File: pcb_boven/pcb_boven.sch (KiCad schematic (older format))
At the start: 30 parts, among them U1 miniIMU-9_v6, U2 openMV_M7_R2

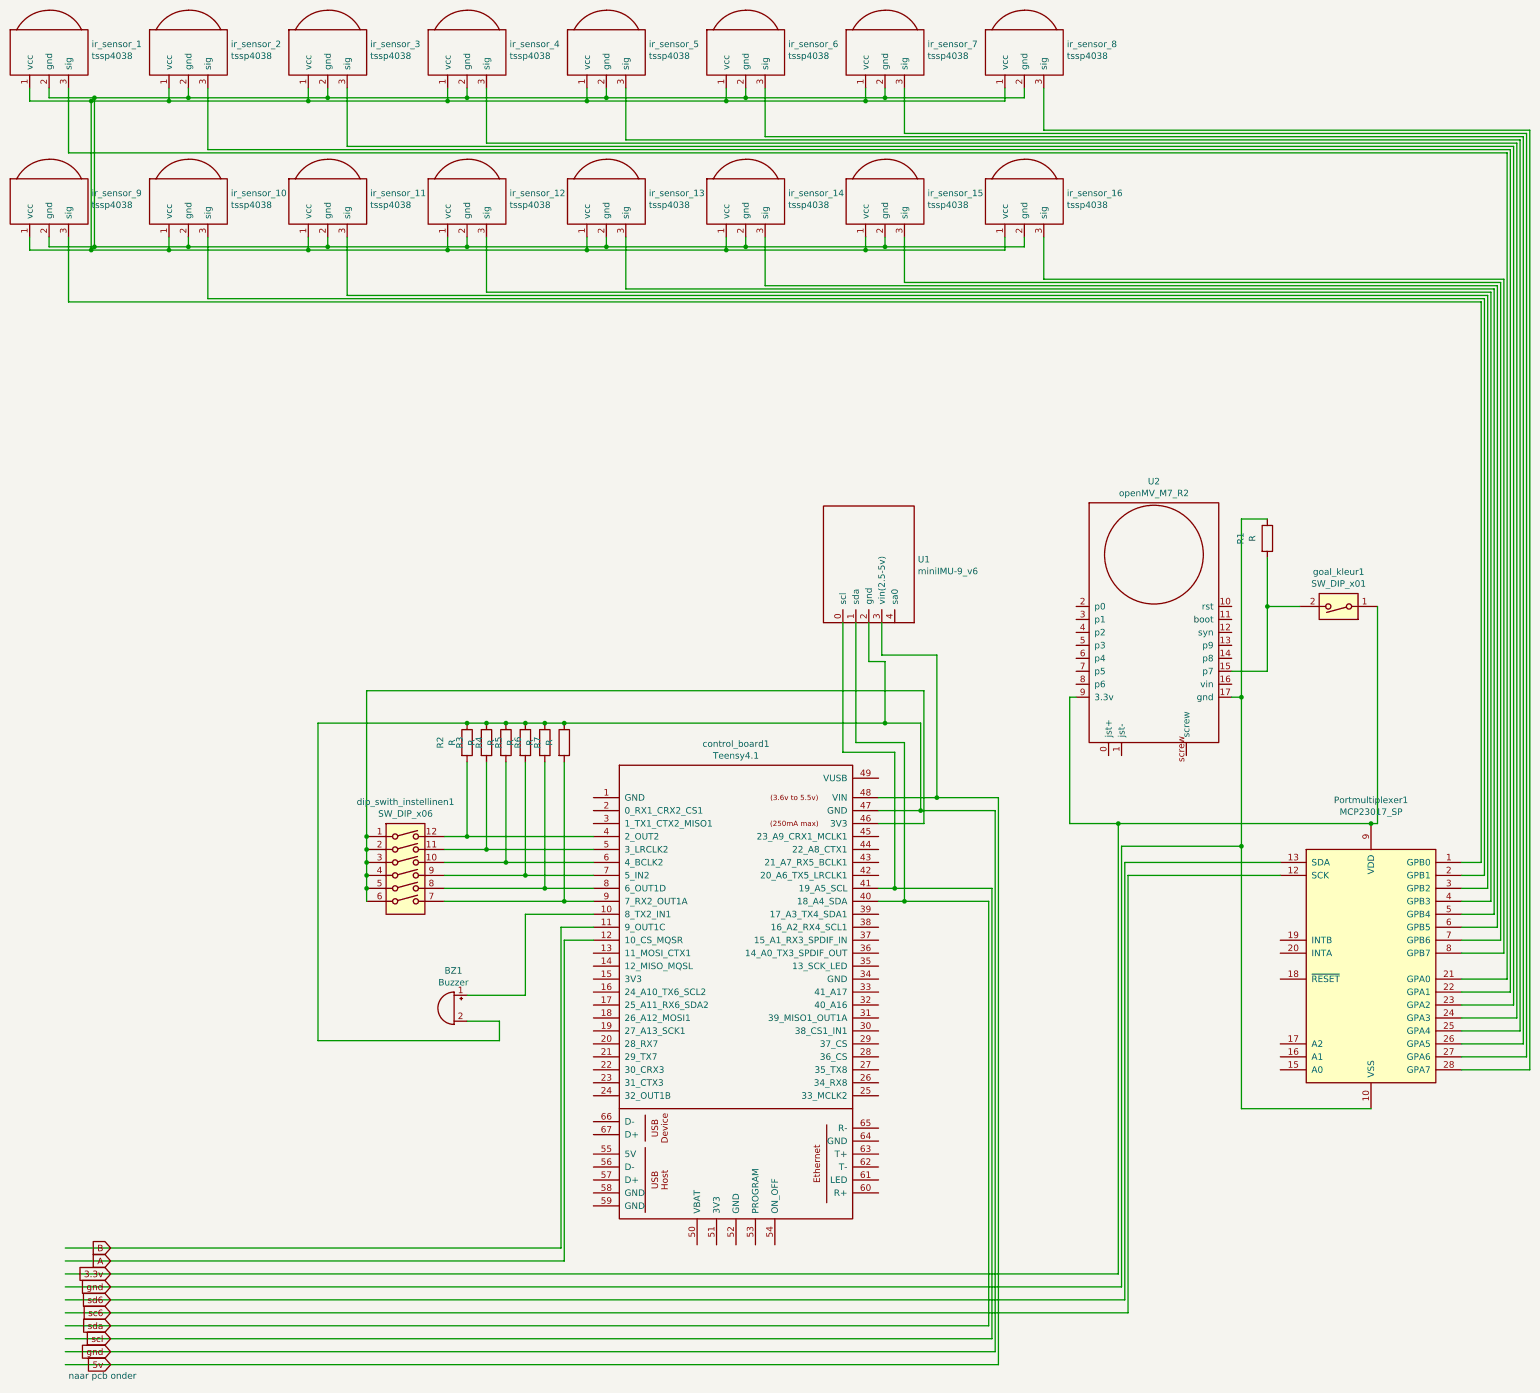
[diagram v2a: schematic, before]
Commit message: pcb onder gemaakt
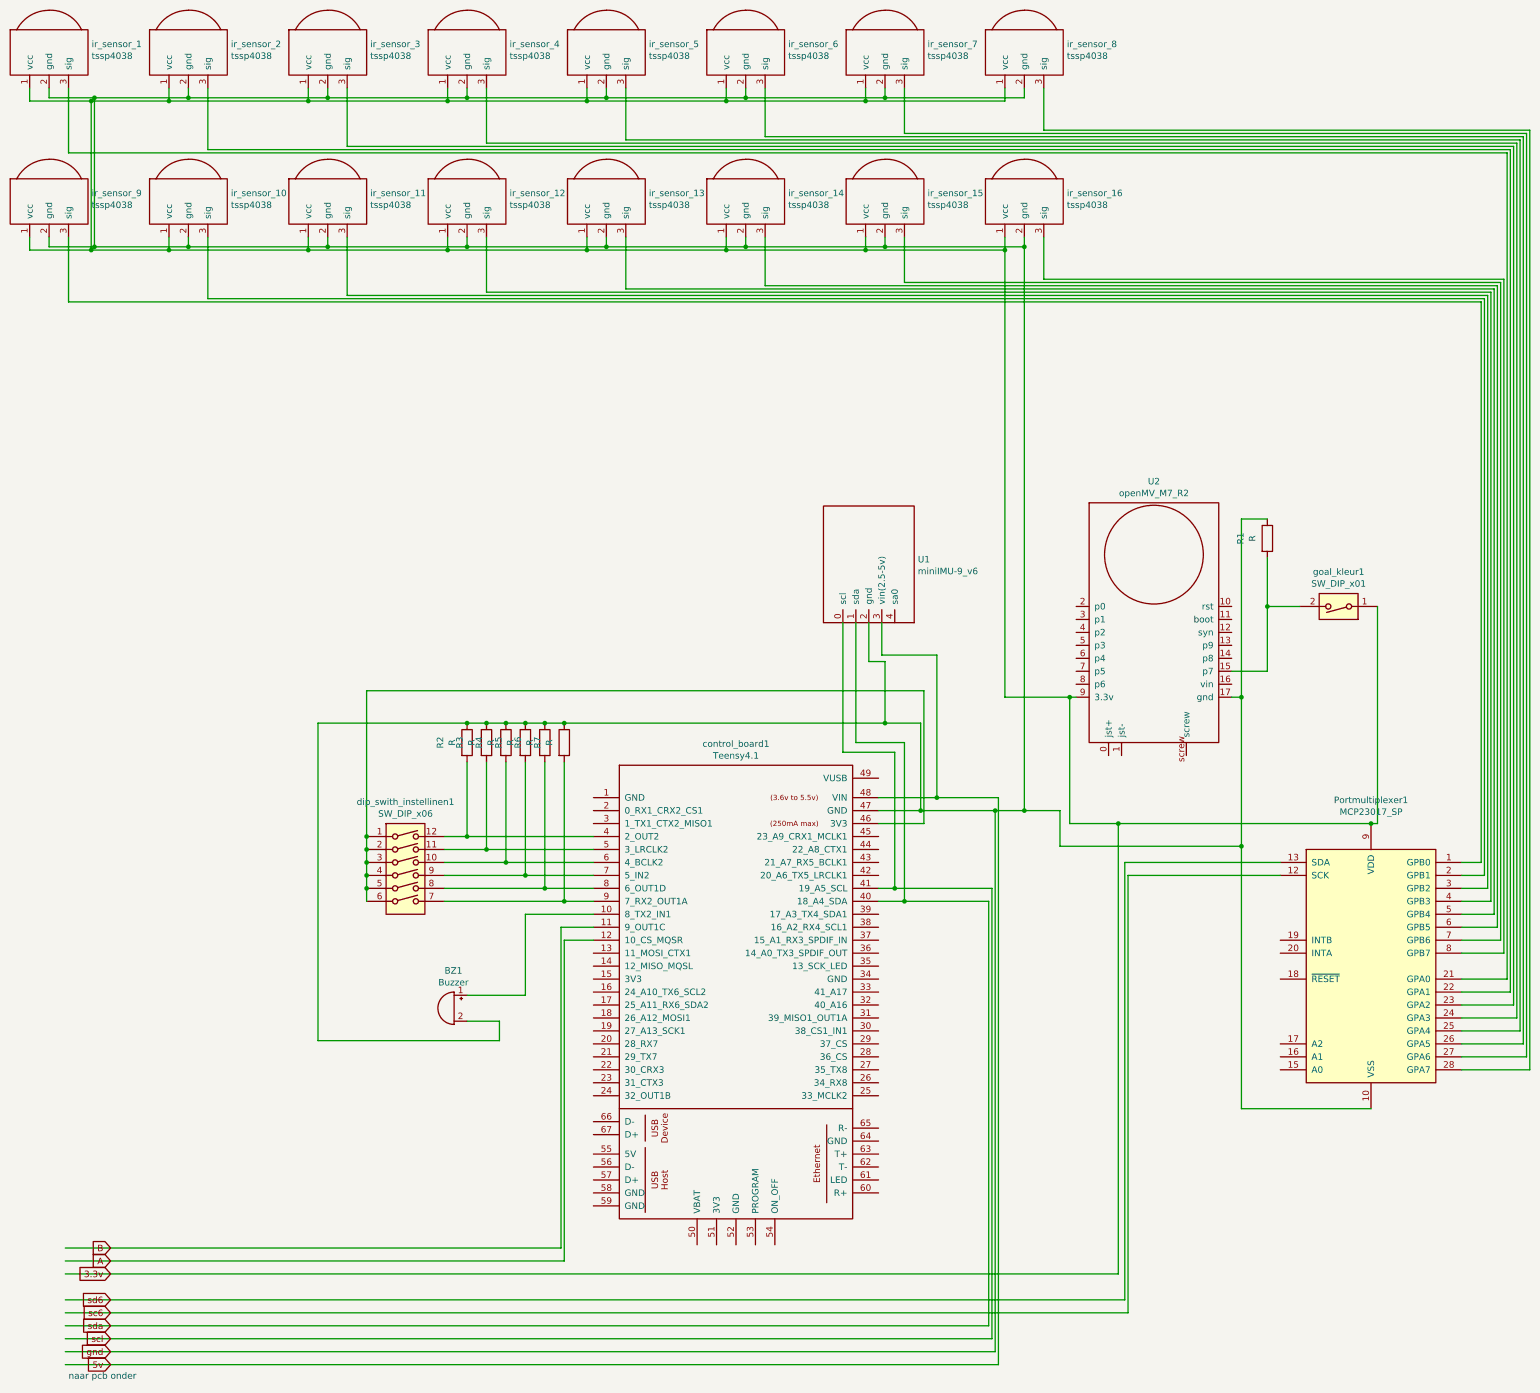
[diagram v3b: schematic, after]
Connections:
- wire segments 234 -> 238
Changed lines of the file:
@@
 	10025 5825 10025 6975
-Wire Wire Line
-	10025 6975 9100 6975
-Wire Wire Line
-	9100 6975 9100 10375
-Wire Wire Line
-	9100 10375 950  10375
 Wire Wire Line
 	9075 10275 9075 6800
@@
 Text GLabel 1300 10275 0    50   Input ~ 0
 3.3v
-Text GLabel 1300 10375 0    50   Input ~ 0
-gnd
 Wire Wire Line
 	11025 6800 9075 6800
@@
 Wire Wire Line
 	4775 10075 950  10075
+Wire Wire Line
+	8125 6700 8350 6700
+Wire Wire Line
+	8625 6700 8625 6975
+Wire Wire Line
+	8625 6975 10025 6975
+Connection ~ 8125 6700
+Wire Wire Line
+	8350 2350 8350 6700
+Connection ~ 8350 2350
+Connection ~ 8350 6700
+Wire Wire Line
+	8350 6700 8625 6700
+Wire Wire Line
+	8200 2375 8200 5825
+Wire Wire Line
+	8200 5825 8700 5825
+Connection ~ 8200 2375
+Connection ~ 8700 5825
 $EndSCHEMATC
